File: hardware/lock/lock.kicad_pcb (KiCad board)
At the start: 2 copper layers, 64 x 23 mm, 50 parts, among them J2 I2C JST-PH RA, J3 SOLENOID 12V, J4 UPDI PROG, J5 SERVO S/V+/GND, J6 HALL DOOR, J7 HALL BOLT, J8 SERVO2 S/V+/GND, Q1 AO3400A, Q2 AO3400A, Q3 AO3401A, Q4 AO3400A, Q5 AO3400A, U1 ATtiny1616, U2 MT3608

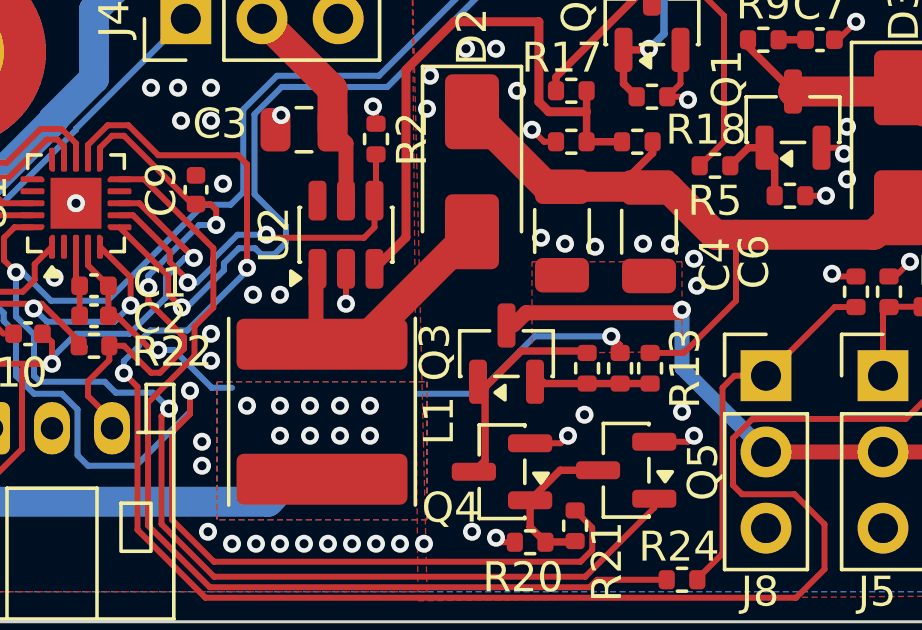
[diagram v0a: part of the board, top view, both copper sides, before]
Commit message: lock: PCB edits — DRC/ERC cleanup in progress
Co-Authored-By: Claude Opus 4.8 (1M context) <noreply@anthropic.com>
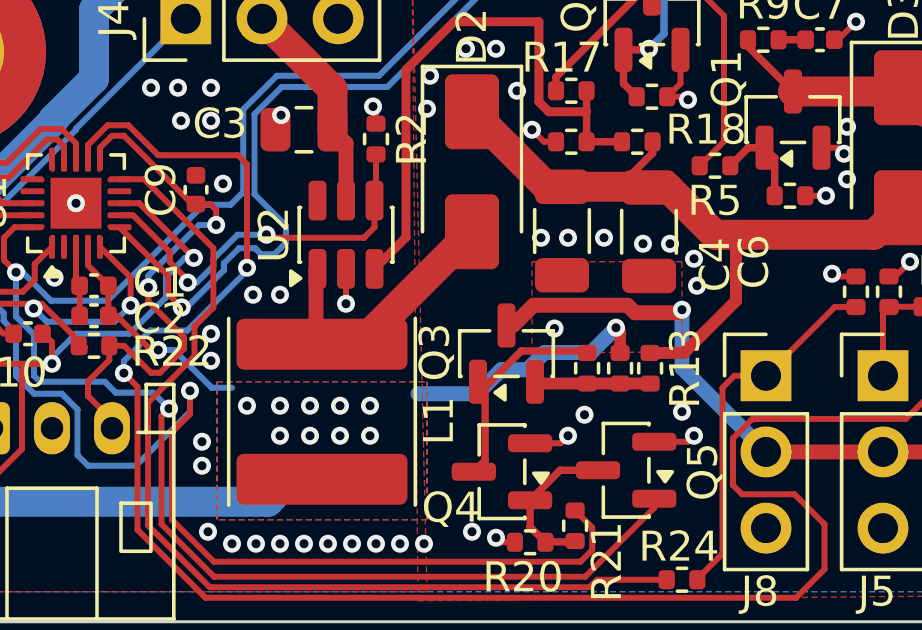
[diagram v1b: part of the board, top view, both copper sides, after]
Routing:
- net /MCU/HALL_DOOR: track 28.3 -> 27.8 mm
- net GND: vias 74 -> 75
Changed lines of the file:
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@@
+	)
+	(via
+		(at 130.75047 71.225)
+		(size 0.6)
+		(drill 0.3)
+		(layers "F.Cu" "B.Cu")
+		(free yes)
+		(net "GND")
 	)
 	(via
@@
 	)
 	(via
-		(at 131.1 68.4)
+		(at 131.2 68.2)
 		(size 0.6)
 		(drill 0.3)
@@
 	)
 	(via
-		(at 132.1 68.5)
+		(at 132.4 68.2)
 		(size 0.6)
 		(drill 0.3)
@@
 	)
 	(segment
-		(start 118.366486 68.507526)
-		(end 118.729265 68.870305)
-		(width 0.2)
-		(layer "F.Cu")
-		(net "/MCU/HALL_DOOR")
-	)
-	(segment
 		(start 110.97471 72.48471)
 		(end 111.741798 72.48471)
@@
 		(layer "B.Cu")
 		(net "/MCU/HALL_DOOR")
+	)
+	(segment
+		(start 129.3875 71.1125)
+		(end 130.05 70.45)
+		(width 0.5)
+		(layer "F.Cu")
+		(net "/DRV/VSERVO")
 	)
 	(segment
@@
 	)
 	(segment
+		(start 130.05 70.45)
+		(end 133.181371 70.45)
+		(width 0.5)
+		(layer "F.Cu")
+		(net "/DRV/VSERVO")
+	)
+	(segment
+		(start 133.181371 70.45)
+		(end 133.431371 70.7)
+		(width 0.5)
+		(layer "F.Cu")
+		(net "/DRV/VSERVO")
+	)
+	(segment
+		(start 145.06 75.34)
+		(end 141.7 75.34)
+		(width 0.5)
+		(layer "F.Cu")
+		(net "/DRV/VSERVO")
+	)
+	(segment
+		(start 141.7 75.34)
+		(end 137.8 75.34)
+		(width 0.5)
+		(layer "F.Cu")
+		(net "/DRV/VSERVO")
+	)
+	(segment
+		(start 133.431371 70.7)
+		(end 134.9 70.7)
+		(width 0.5)
+		(layer "F.Cu")
+		(net "/DRV/VSERVO")
+	)
+	(segment
 		(start 134.9 70.7)
 		(end 135 70.6)
@@
 		(net "/DRV/VSERVO")
 	)
-	(segment
-		(start 145.06 75.34)
-		(end 141.7 75.34)
-		(width 0.5)
-		(layer "F.Cu")
-		(net "/DRV/VSERVO")
-	)
-	(segment
-		(start 129.8 70.7)
-		(end 134.9 70.7)
-		(width 0.5)
-		(layer "F.Cu")
-		(net "/DRV/VSERVO")
-	)
-	(segment
-		(start 141.7 75.34)
-		(end 137.8 75.34)
-		(width 0.5)
-		(layer "F.Cu")
-		(net "/DRV/VSERVO")
-	)
-	(segment
-		(start 129.3875 71.1125)
-		(end 129.8 70.7)
-		(width 0.5)
-		(layer "F.Cu")
-		(net "/DRV/VSERVO")
-	)
 	(via
 		(at 135 70.6)
@@
 		(start 136.8 70.3)
 		(end 136.8 68.1)
-		(width 0.2)
+		(width 0.4)
 		(layer "F.Cu")
 		(net "VSOL")
@@
 		(start 135.06 72.04)
 		(end 136.8 70.3)
-		(width 0.2)
+		(width 0.4)
 		(layer "F.Cu")
 		(net "VSOL")
@@
 		(start 133.9375 72.04)
 		(end 135.06 72.04)
-		(width 0.2)
+		(width 0.4)
 		(layer "F.Cu")
 		(net "VSOL")
@@
 	)
 	(segment
-		(start 132.9375 71.770001)
-		(end 132.65534 71.487841)
-		(width 0.2)
+		(start 132.9375 72.04)
+		(end 132.9375 71.3375)
+		(width 0.4)
 		(layer "F.Cu")
 		(net "VCC")
@@
 		(start 115.2 69.12)
 		(end 115.88 69.8)
-		(width 0.2)
-		(layer "F.Cu")
-		(net "VCC")
-	)
-	(segment
-		(start 132.65534 71.487841)
-		(end 132.643531 71.487841)
 		(width 0.2)
 		(layer "F.Cu")
@@
 	)
 	(segment
-		(start 132.9375 72.04)
-		(end 132.9375 71.770001)
-		(width 0.2)
-		(layer "F.Cu")
-		(net "VCC")
-	)
-	(segment
 		(start 123.35 63.25)
 		(end 123.35 64.6)
@@
 		(net "VCC")
 	)
+	(segment
+		(start 132.9375 71.3375)
+		(end 132.8 71.2)
+		(width 0.2)
+		(layer "F.Cu")
+		(net "VCC")
+	)
 	(via
 		(at 122.6 73.8)
@@
 	)
 	(via
-		(at 132.643531 71.487841)
+		(at 132.8 71.2)
 		(size 0.6)
 		(drill 0.3)
@@
 	)
 	(segment
+		(start 130.419099 72.025)
+		(end 131.975 72.025)
+		(width 0.5)
+		(layer "B.Cu")
+		(net "VCC")
+	)
+	(segment
 		(start 118.063861 71.942175)
 		(end 117.542173 71.942175)
@@
 	)
 	(segment
+		(start 126.2 73.4)
+		(end 128.175516 73.4)
+		(width 0.5)
+		(layer "B.Cu")
+		(net "VCC")
+	)
+	(segment
 		(start 115.4 60.6)
 		(end 116.6 59.4)
@@
 	)
 	(segment
-		(start 128.175516 73.4)
-		(end 130.087675 71.487841)
-		(width 0.2)
-		(layer "B.Cu")
-		(net "VCC")
-	)
-	(segment
 		(start 109.175 66.4)
 		(end 110.4 66.4)
@@
 	)
 	(segment
-		(start 126.2 73.4)
-		(end 128.175516 73.4)
-		(width 0.2)
+		(start 131.975 72.025)
+		(end 132.8 71.2)
+		(width 0.5)
+		(layer "B.Cu")
+		(net "VCC")
+	)
+	(segment
+		(start 129.844099 72.6)
+		(end 130.419099 72.025)
+		(width 0.5)
 		(layer "B.Cu")
 		(net "VCC")
@@
 	)
 	(segment
-		(start 130.087675 71.487841)
-		(end 132.643531 71.487841)
-		(width 0.2)
-		(layer "B.Cu")
-		(net "VCC")
-	)
-	(segment
 		(start 119.321686 73.2)
 		(end 118.063861 71.942175)
@@
 	)
 	(segment
+		(start 128.175516 73.4)
+		(end 128.975516 72.6)
+		(width 0.5)
+		(layer "B.Cu")
+		(net "VCC")
+	)
+	(segment
+		(start 128.975516 72.6)
+		(end 129.844099 72.6)
+		(width 0.5)
+		(layer "B.Cu")
+		(net "VCC")
+	)
+	(segment
 		(start 131.7725 71.975)
 		(end 129.642696 71.975)
@@
 		(start 132.9375 73.06)
 		(end 131.8375 73.06)
-		(width 0.25)
+		(width 0.4)
 		(layer "F.Cu")
 		(net "/DRV/VSERVO_SRC")
@@
 		(start 133.9375 73.06)
 		(end 132.9375 73.06)
-		(width 0.25)
+		(width 0.4)
 		(layer "F.Cu")
 		(net "/DRV/VSERVO_SRC")
@@
 		(start 131.8375 73.06)
 		(end 130.41 73.06)
-		(width 0.25)
+		(width 0.4)
 		(layer "F.Cu")
 		(net "/DRV/VSERVO_SRC")
@@
 			(thermal_gap 0.5)
 			(thermal_bridge_width 0.5)
-			(smoothing chamfer)
+			(smoothing fillet)
+			(radius 1)
 			(island_removal_mode 0)
 		)
@@
 			(thermal_gap 0.5)
 			(thermal_bridge_width 0.5)
-			(smoothing chamfer)
+			(smoothing fillet)
+			(radius 1)
 			(island_removal_mode 0)
 		)
